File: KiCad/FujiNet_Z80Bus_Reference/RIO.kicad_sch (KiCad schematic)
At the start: 17 parts, among them IC19 7432N, IC2 7404N, IC20 7408N, IC4 7432N, IC5 7408N

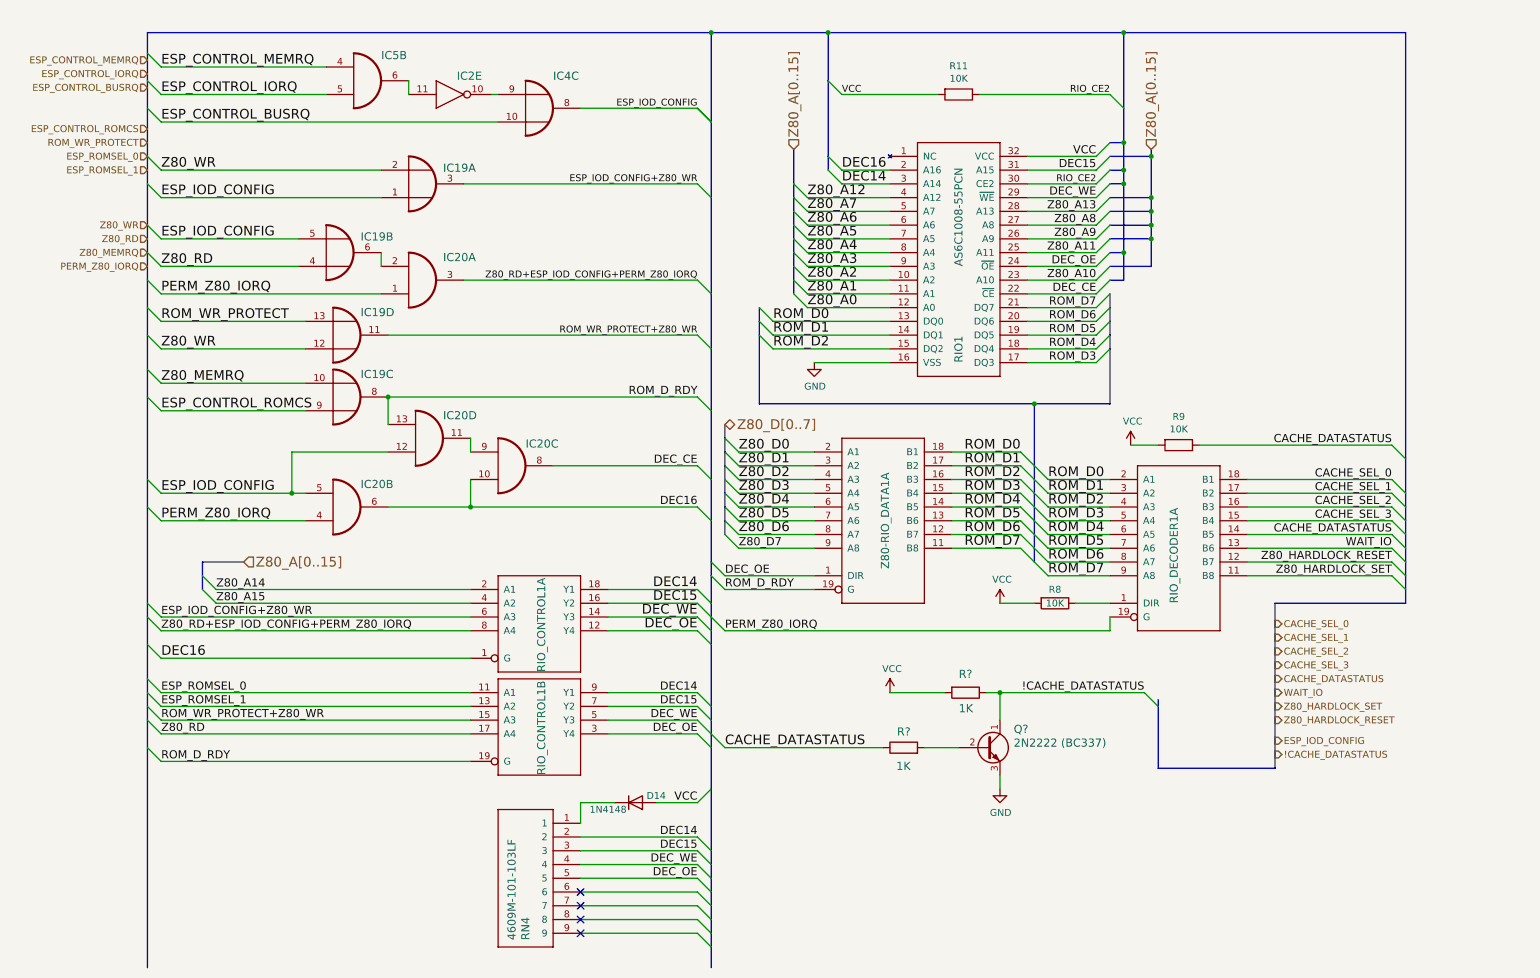
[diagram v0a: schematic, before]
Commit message: Massive fix to KiCad Labels
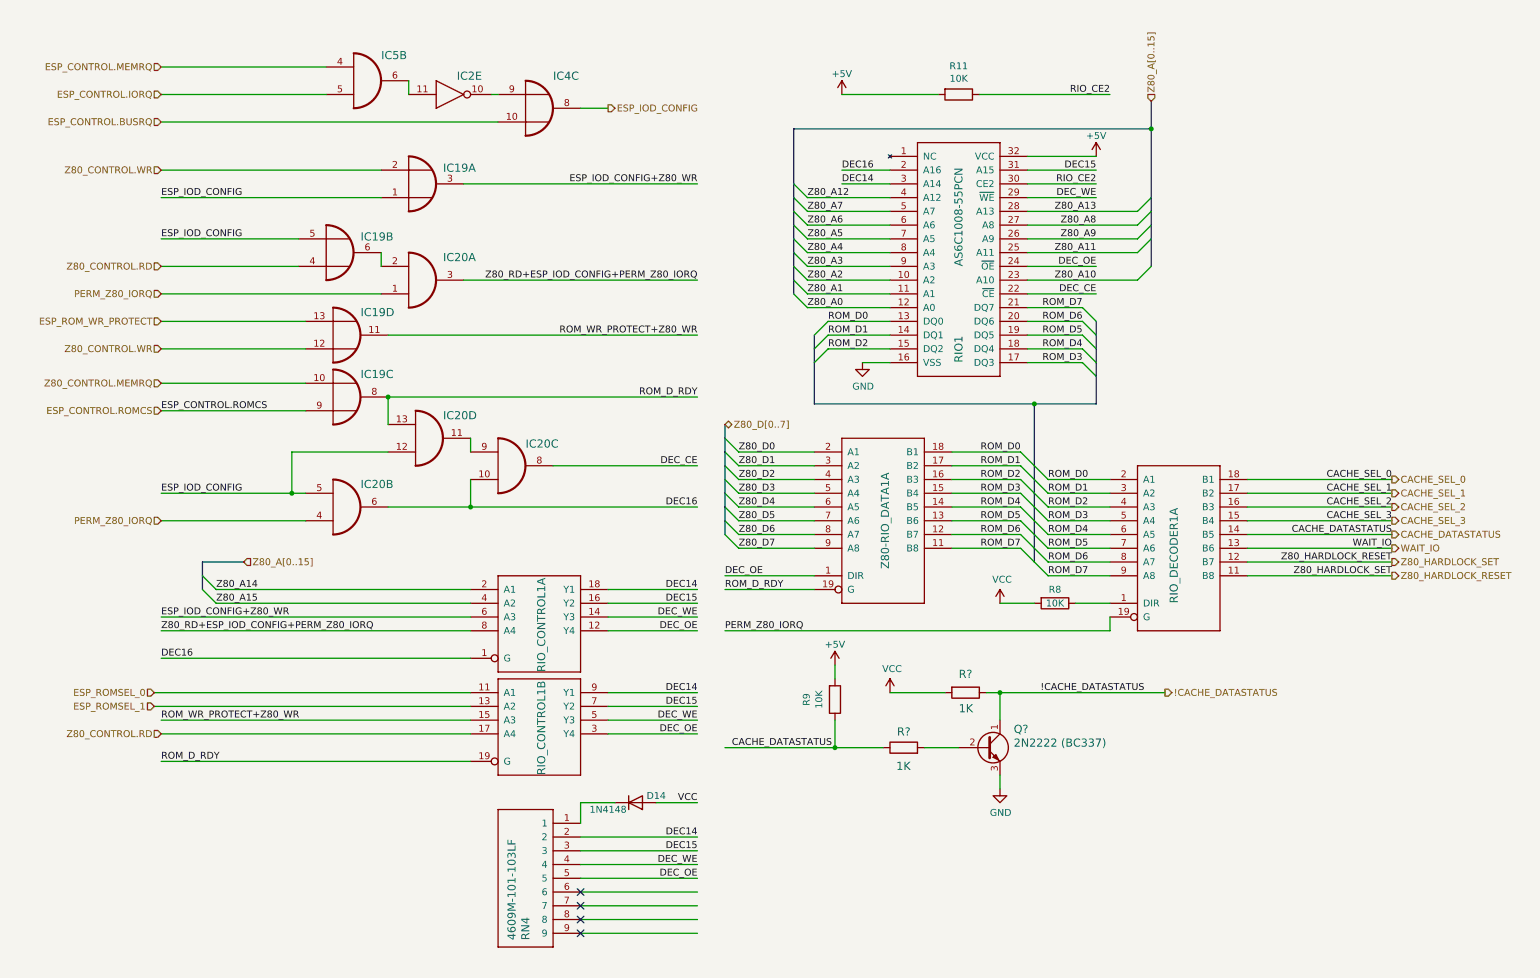
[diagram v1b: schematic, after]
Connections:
- net Z80_HARDLOCK_SET is gone; now on net Z80_HARDLOCK_RESET: RIO_DECODER1.11 (B8)
- net VCC: no longer R11.2, R9.2, RIO1.32 (VCC)
- net ESP_CONTROL_BUSRQ renamed ESP_CONTROL.BUSRQ
- net ESP_CONTROL_IORQ renamed ESP_CONTROL.IORQ
- net ESP_CONTROL_MEMRQ renamed ESP_CONTROL.MEMRQ
- net ESP_CONTROL_ROMCS renamed ESP_CONTROL.ROMCS
- net ROM_WR_PROTECT renamed ESP_ROM_WR_PROTECT
- net Z80_MEMRQ renamed Z80_CONTROL.MEMRQ
- net Z80_RD renamed Z80_CONTROL.RD
- net Z80_WR renamed Z80_CONTROL.WR
- new net +5V: R11.2, R9.2, RIO1.32 (VCC)
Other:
- moved on the sheet: R9
